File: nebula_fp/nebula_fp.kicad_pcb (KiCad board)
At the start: 2 copper layers, 62 x 62 mm, 4 parts

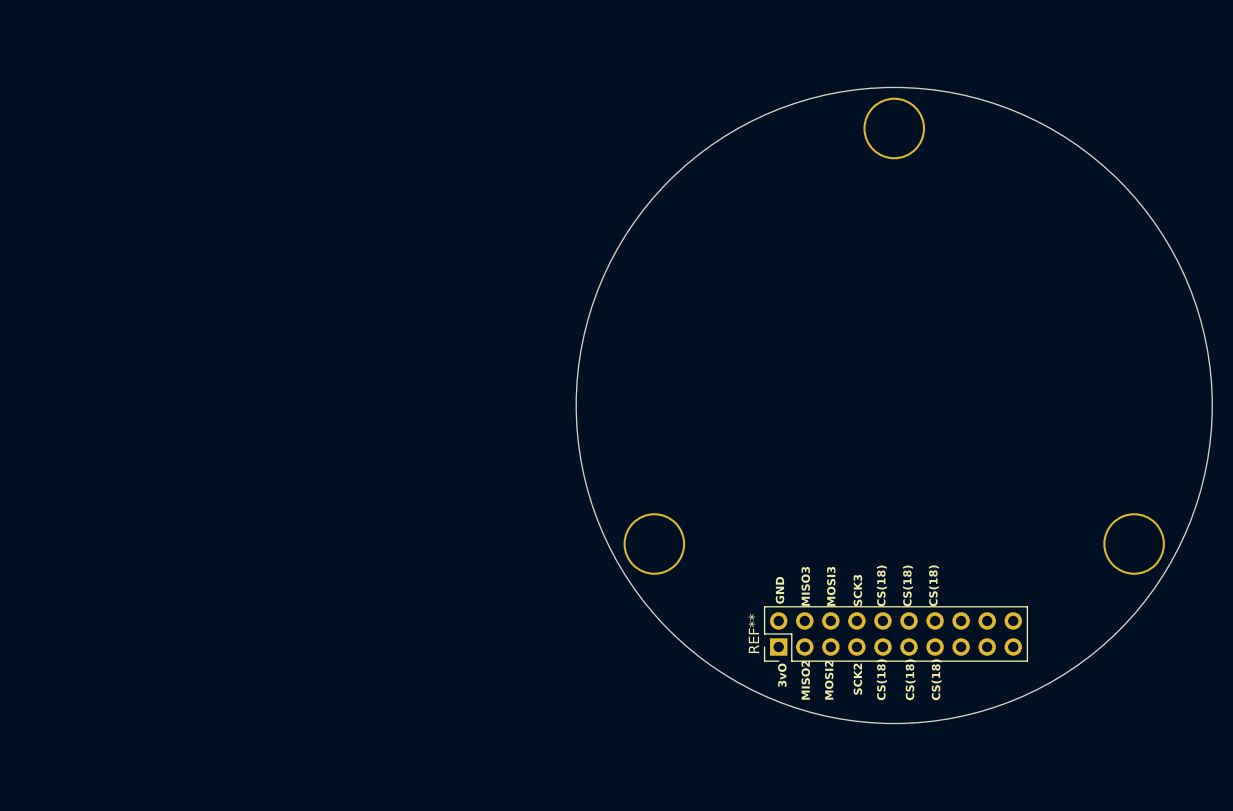
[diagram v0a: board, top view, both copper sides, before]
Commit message: update nebula FP
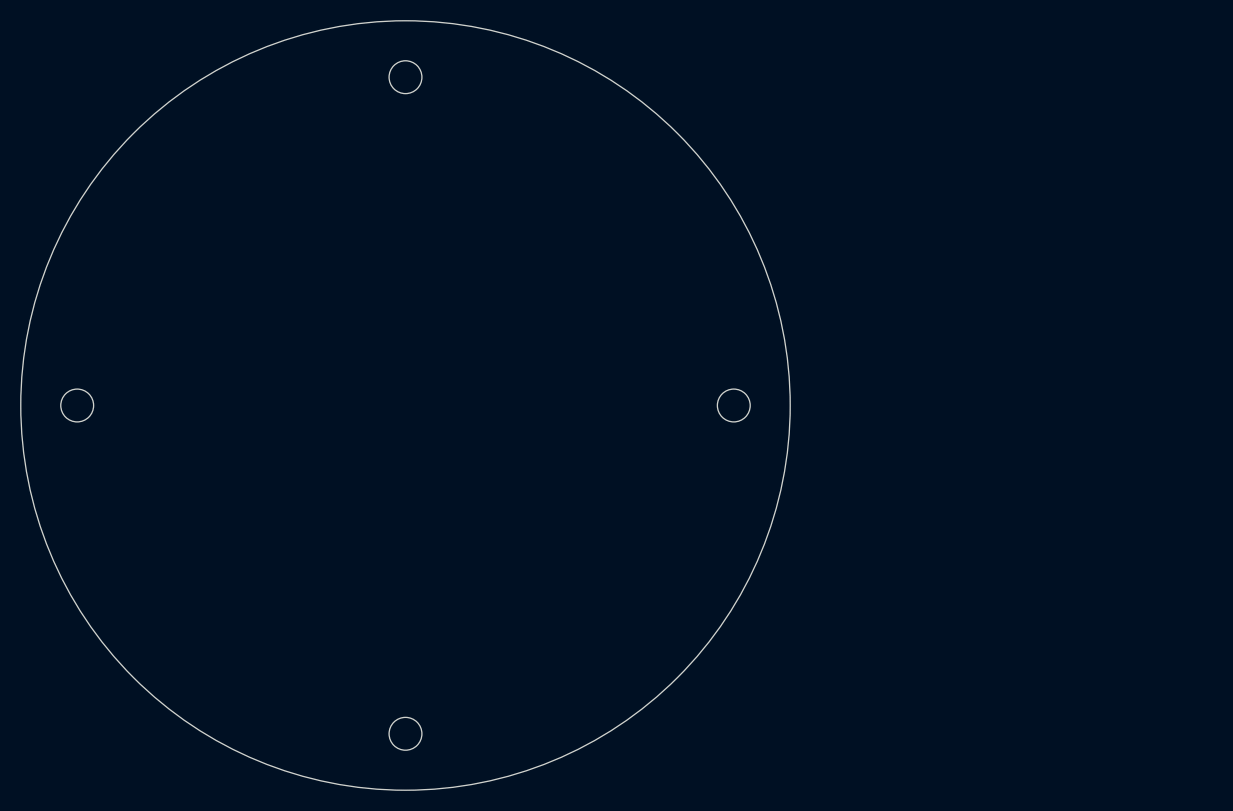
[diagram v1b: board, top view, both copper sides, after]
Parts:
- removed the REF** at (156.4, 123.5)
- removed the REF** at (144.3, 113.5)
- removed the REF** at (191.0, 113.5)
- removed the REF** at (167.6, 73.0)
- added REF**: MountingHole_3.2mm_M3, MountingHole:MountingHole_3.2mm_M3, F.Cu at (120.0, 132.0)
- added REF**: MountingHole_3.2mm_M3, MountingHole:MountingHole_3.2mm_M3, F.Cu at (120.0, 68.0)
- added REF**: MountingHole_3.2mm_M3, MountingHole:MountingHole_3.2mm_M3, F.Cu at (152.0, 100.0)
- added REF**: MountingHole_3.2mm_M3, MountingHole:MountingHole_3.2mm_M3, F.Cu at (88.0, 100.0)
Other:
- board size 62 x 62 mm -> 75 x 75 mm
- board text removed: "3vO"
- board text removed: "CS(18)"
- board text removed: "GND"
- board text removed: "MISO2"
- board text removed: "MISO3"
- board text removed: "MOSI2"
- board text removed: "MOSI3"
- board text removed: "SCK2"
- board text removed: "SCK3"
